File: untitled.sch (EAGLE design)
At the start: 22 parts, among them T1 E13005, T2 2N3565

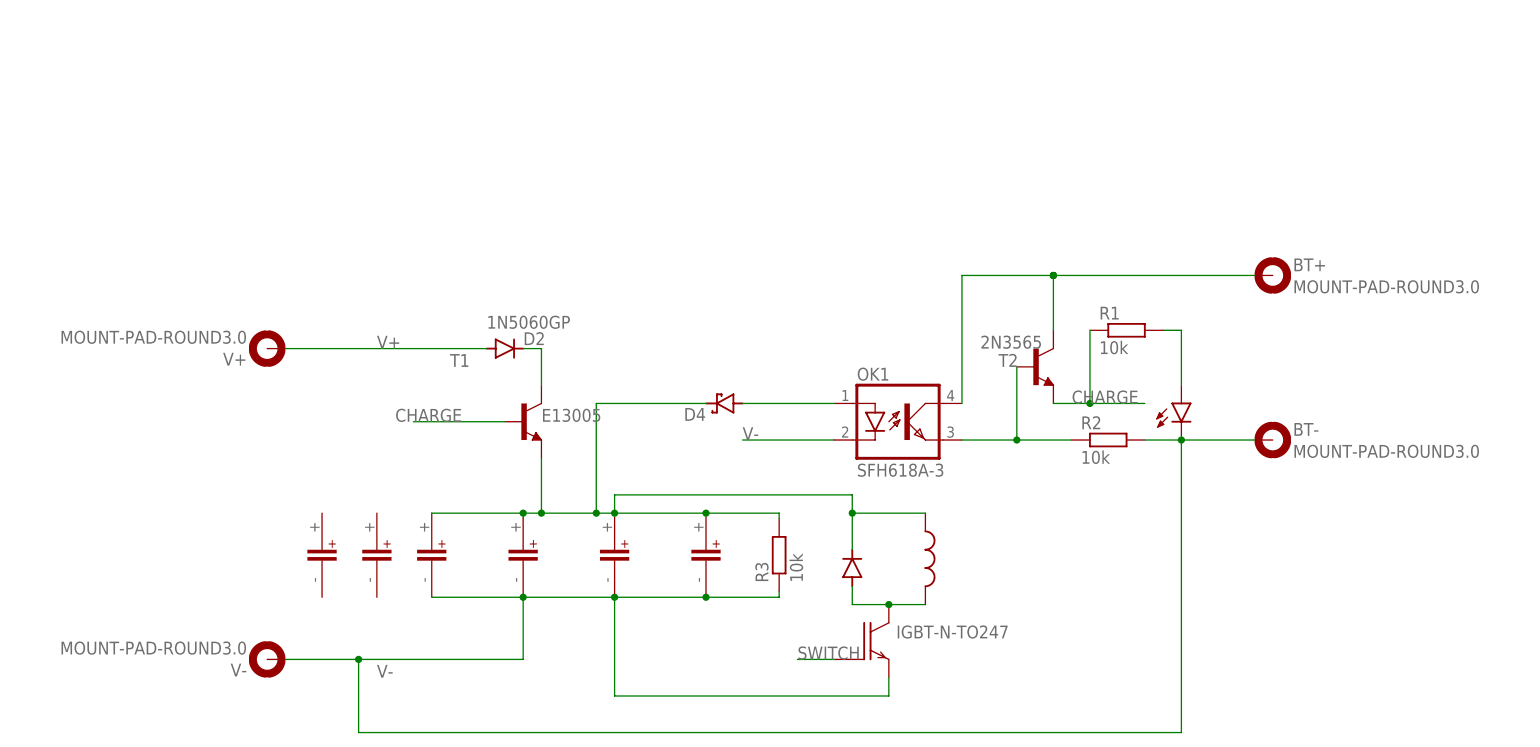
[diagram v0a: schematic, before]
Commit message: add
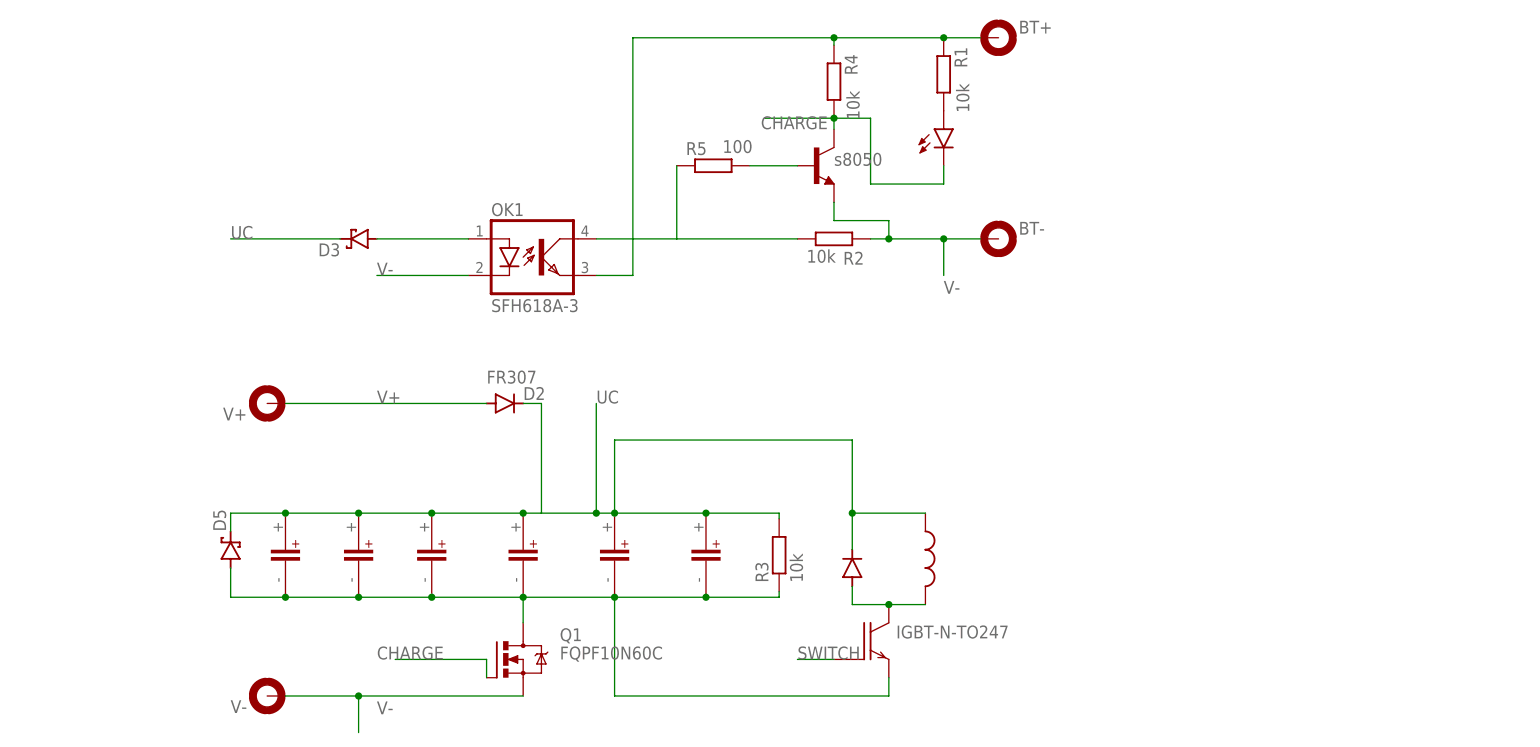
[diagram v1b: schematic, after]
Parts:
- removed D4: (no value), zetex:DS_E2L
- removed T1: E13005, transistor:2SC1306
- added D3, D5: (no value), zetex:DS_E2L
- added Q1: FQPF10N60C, transistor-power:IRF740
- added R4: 10k, rcl:R-EU_0207/2V
- added R5: 100, rcl:R-EU_0207/2V
- D2: value 1N5060GP -> FR307
- T2: value 2N3565 -> s8050; device transistor:2N3565 -> transistor:2N3704
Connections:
- removed net N$1: D2.C, T1.C
- new net N$10: D5.A, Q1.D, R3.1, U$1.-, U$11.-, U$12.-, U$2.-, U$3.-, U$4.-, U$9.E
- new net UC: D1.C, D2.C, D3.K, D5.K, R3.2, U$1.+, U$11.+, U$12.+, U$2.+, U$3.+, U$4.+, U$6.1
- net CHARGE: now also LED1.C, Q1.G, R4.2, T2.C; no longer R1.1, T1.B, T2.E
- net N$2: now also D3.A; no longer D4.A
- net N$3: now also R5.2, T2.B; no longer D1.C, D4.K, R3.2, T1.E, U$1.+, U$2.+, U$3.+, U$4.+, U$6.1
- net N$5: now also OK1.COL, R5.1; no longer OK1.EMIT, T2.B
- net N$7: now also OK1.EMIT, R1.1, R4.1; no longer OK1.COL, T2.C
- net V-: now also Q1.S, T2.E; no longer LED1.C, R3.1, U$1.-, U$2.-, U$3.-, U$4.-, U$9.E
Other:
- moved on the sheet: BT+, BT-, D2, OK1, R1, R2, V+, V-
